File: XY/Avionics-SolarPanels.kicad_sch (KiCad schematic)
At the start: 37 parts, among them J1 200528-0100, J2 200528-0100

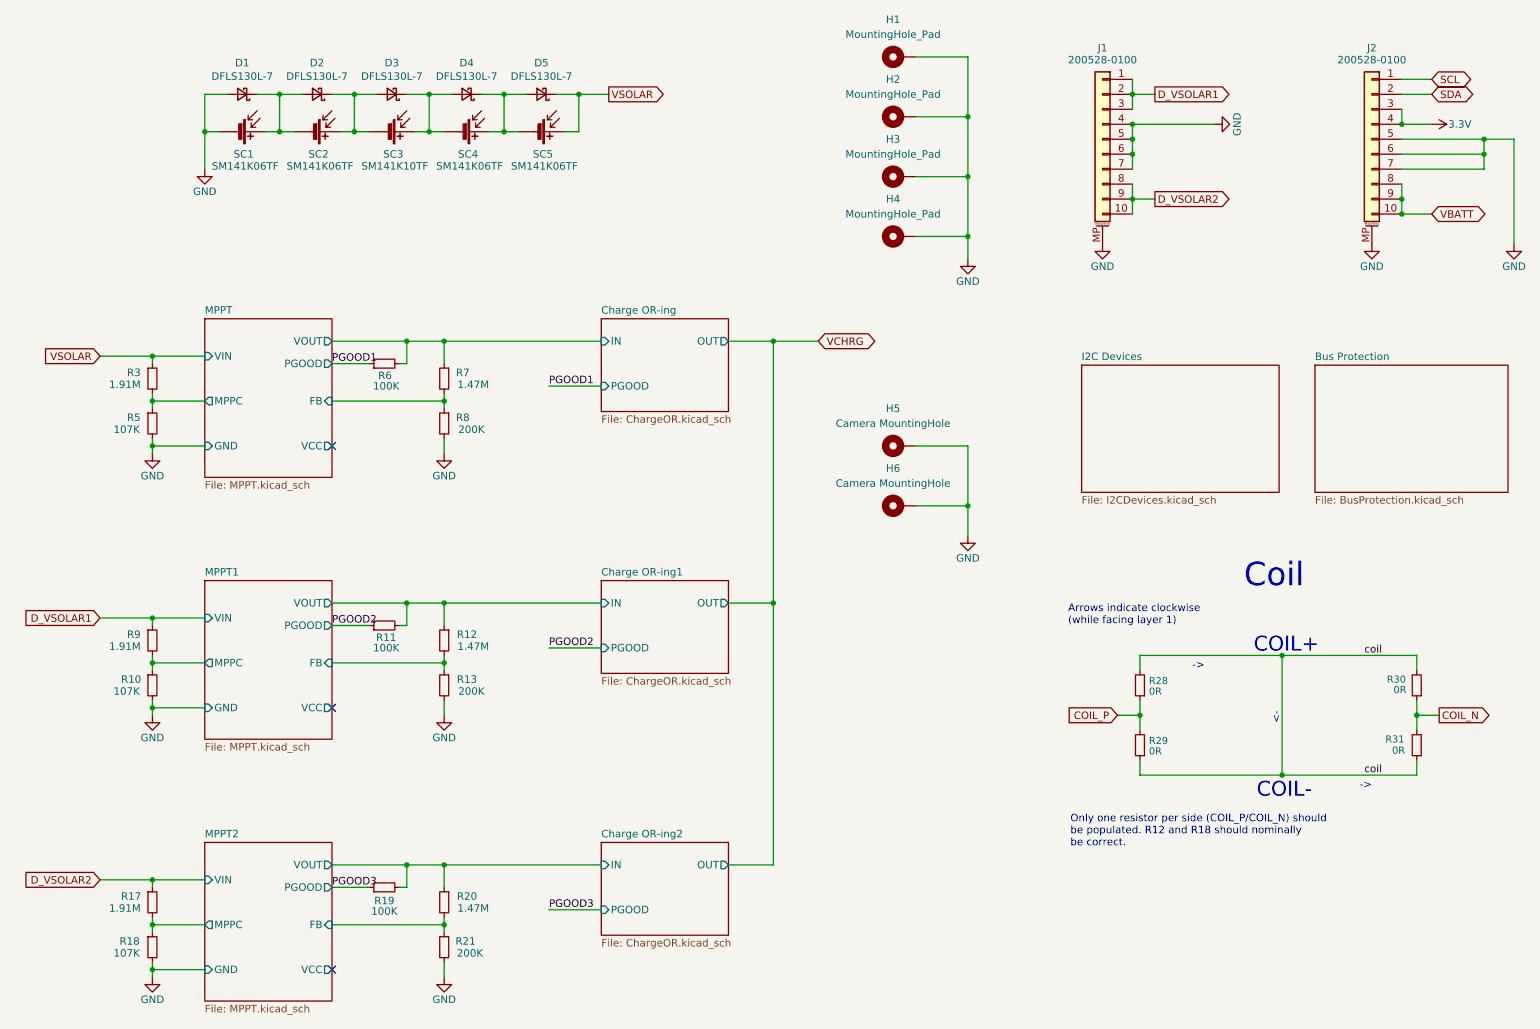
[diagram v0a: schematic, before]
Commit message: Updated XY boards
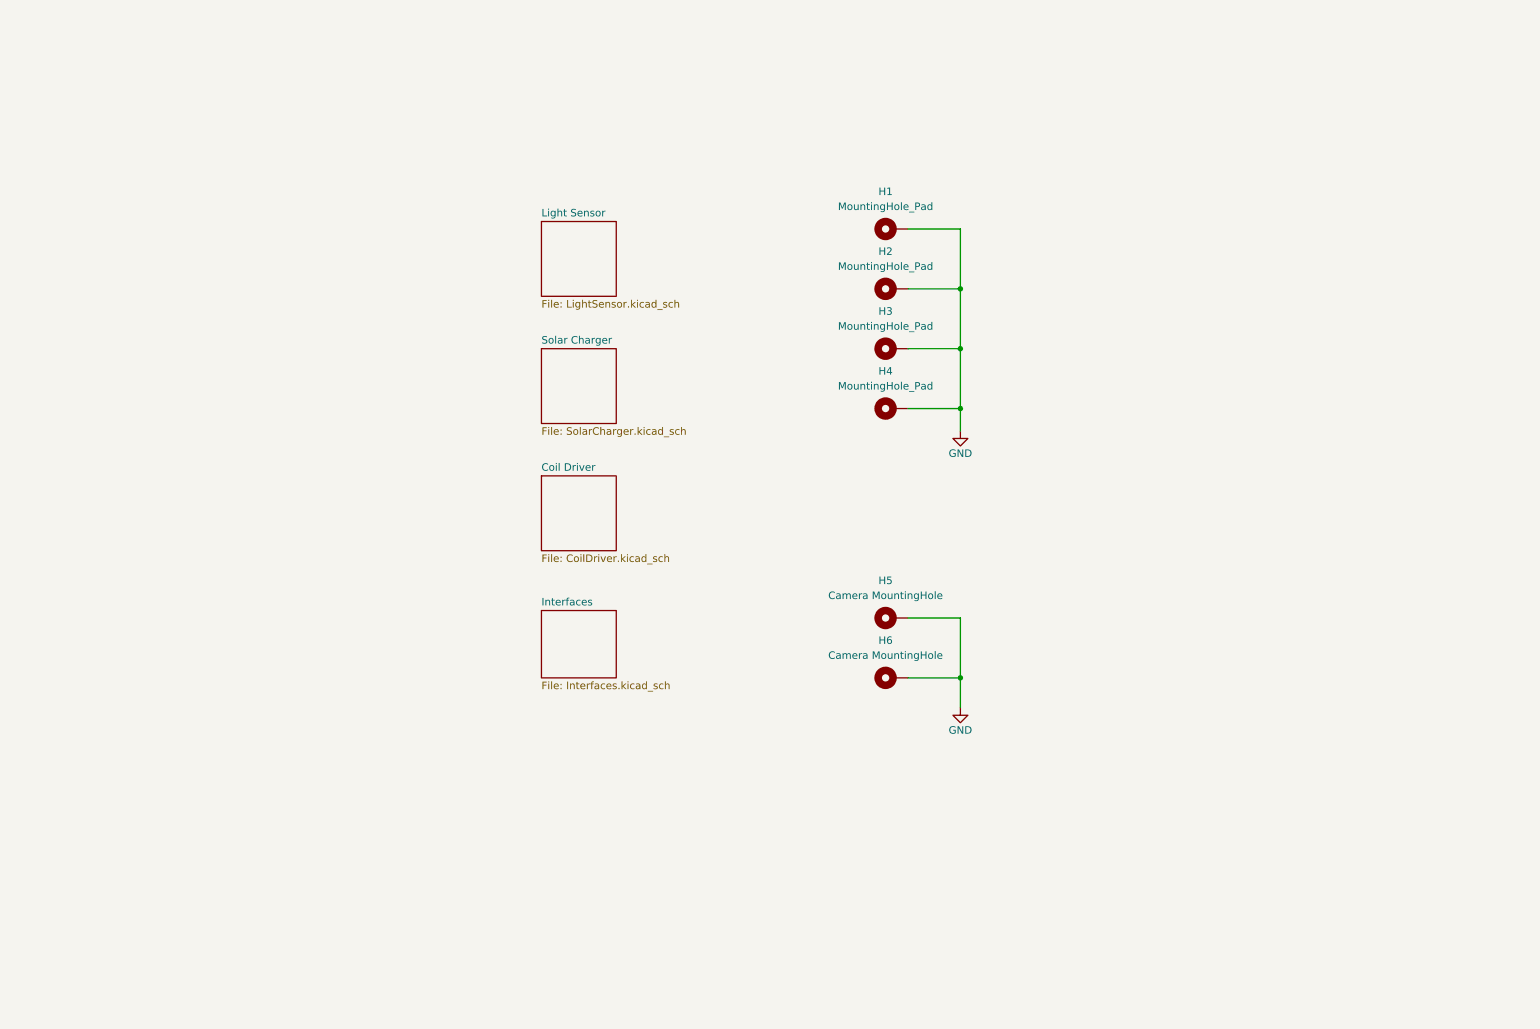
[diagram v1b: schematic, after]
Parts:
- removed D1, D2, D3, D4, D5: DFLS130L-7, Diode_SMD:D_PowerDI-123, symbol Device:D_Schottky_Small
- removed J1, J2: 200528-0100, Connector_FFC-FPC:Molex_200528-0100_1x10-1MP_P1.00mm_Horizontal, symbol Connector_Generic_MountingPin:Conn_01x10_MountingPin
- removed R10, R18, R5: 107K, Resistor_SMD:R_0603_1608Metric, symbol Device:R_Small
- removed R11, R19, R6: 100K, Resistor_SMD:R_0603_1608Metric, symbol Device:R_Small
- removed R12, R20, R7: 1.47M, Resistor_SMD:R_0603_1608Metric, symbol Device:R_Small
- removed R13, R21, R8: 200K, Resistor_SMD:R_0603_1608Metric, symbol Device:R_Small
- removed R17, R3, R9: 1.91M, Resistor_SMD:R_0603_1608Metric, symbol Device:R_Small
- removed R28, R29, R30, R31: 0R, Resistor_SMD:R_0603_1608Metric, symbol Device:R_Small
- removed SC1, SC2, SC4, SC5: SM141K06TF, SolarPanels:SM141K06TF, symbol Device:Solar_Cell
- removed SC3: SM141K10TF, SolarPanels:SM141K10TF, symbol Device:Solar_Cell
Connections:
- no-connect marks 3 -> 0
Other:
- removed sheet Bus Protection
- removed sheet Charge OR-ing
- removed sheet Charge OR-ing1
- removed sheet Charge OR-ing2
- removed sheet I2C Devices
- removed sheet MPPT
- removed sheet MPPT1
- removed sheet MPPT2
- added sheet Coil Driver (CoilDriver.kicad_sch)
- added sheet Interfaces (Interfaces.kicad_sch)
- added sheet Light Sensor (LightSensor.kicad_sch)
- added sheet Solar Charger (SolarCharger.kicad_sch)
- note removed: "->"
- note removed: "<-"
- note removed: "Arrows indicate clockwise (while facing layer 1)"
- note removed: "COIL+"
- note removed: "COIL-"
- note removed: "Coil"
- note removed: "Only one resistor per side (COIL_P/COIL_N) should be populated. R12 and R18 should nominally be correct."
- moved on the sheet: H1, H2, H3, H4, H5, H6
